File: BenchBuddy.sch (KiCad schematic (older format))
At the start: 0 parts

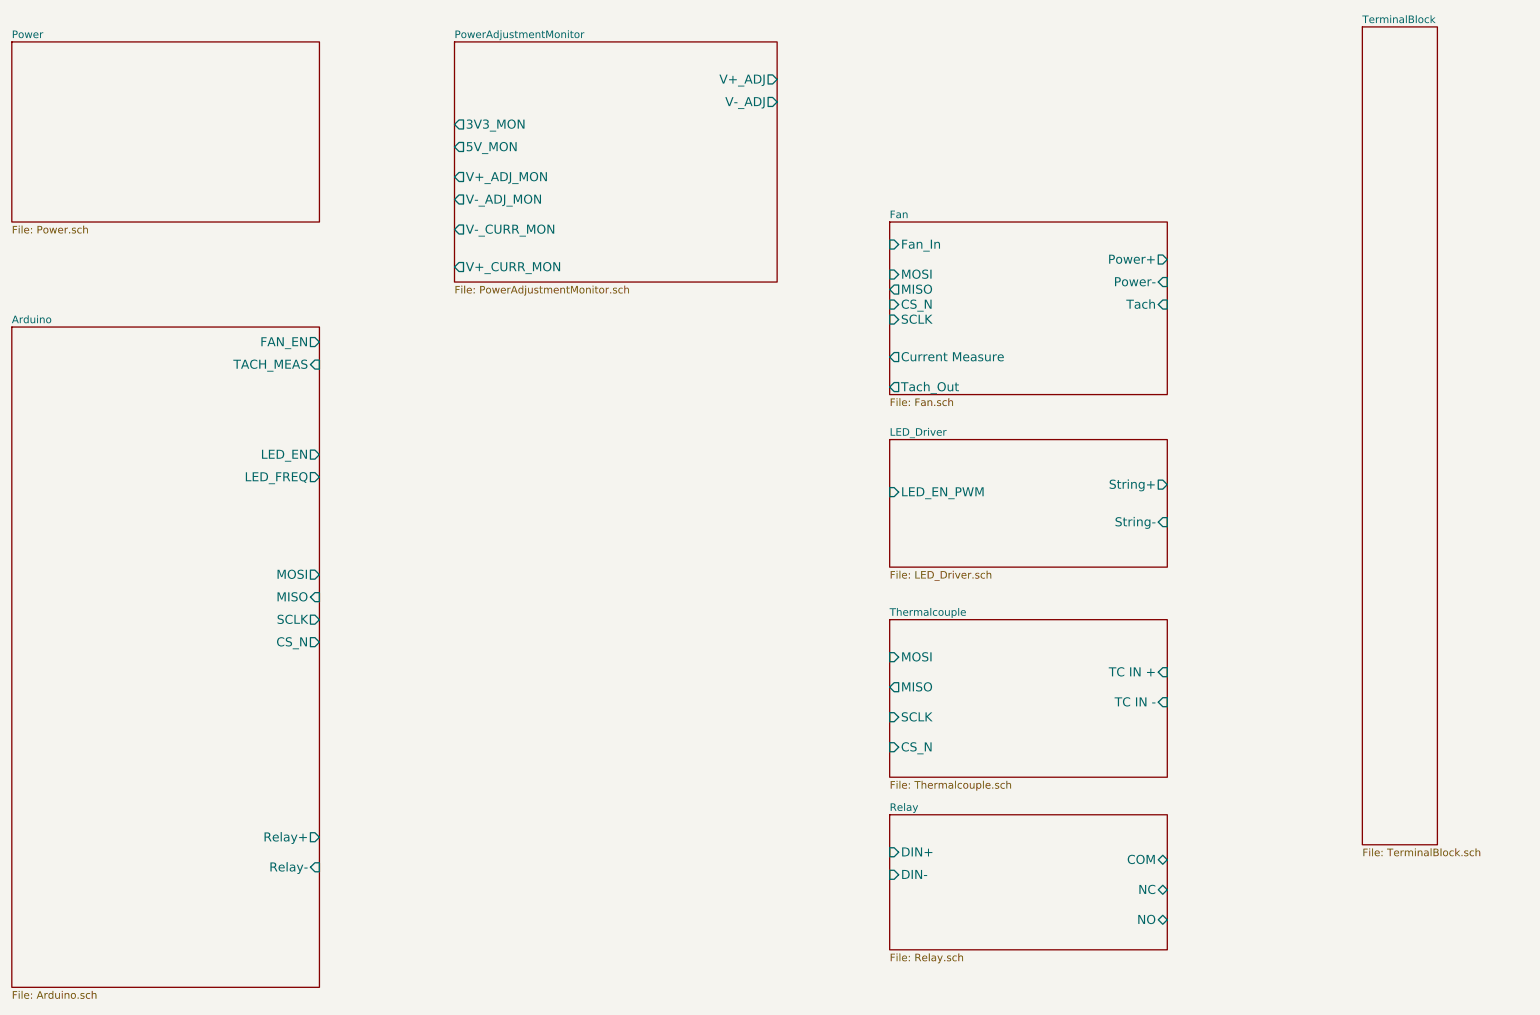
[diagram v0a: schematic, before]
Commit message: arduino module / hooking things up
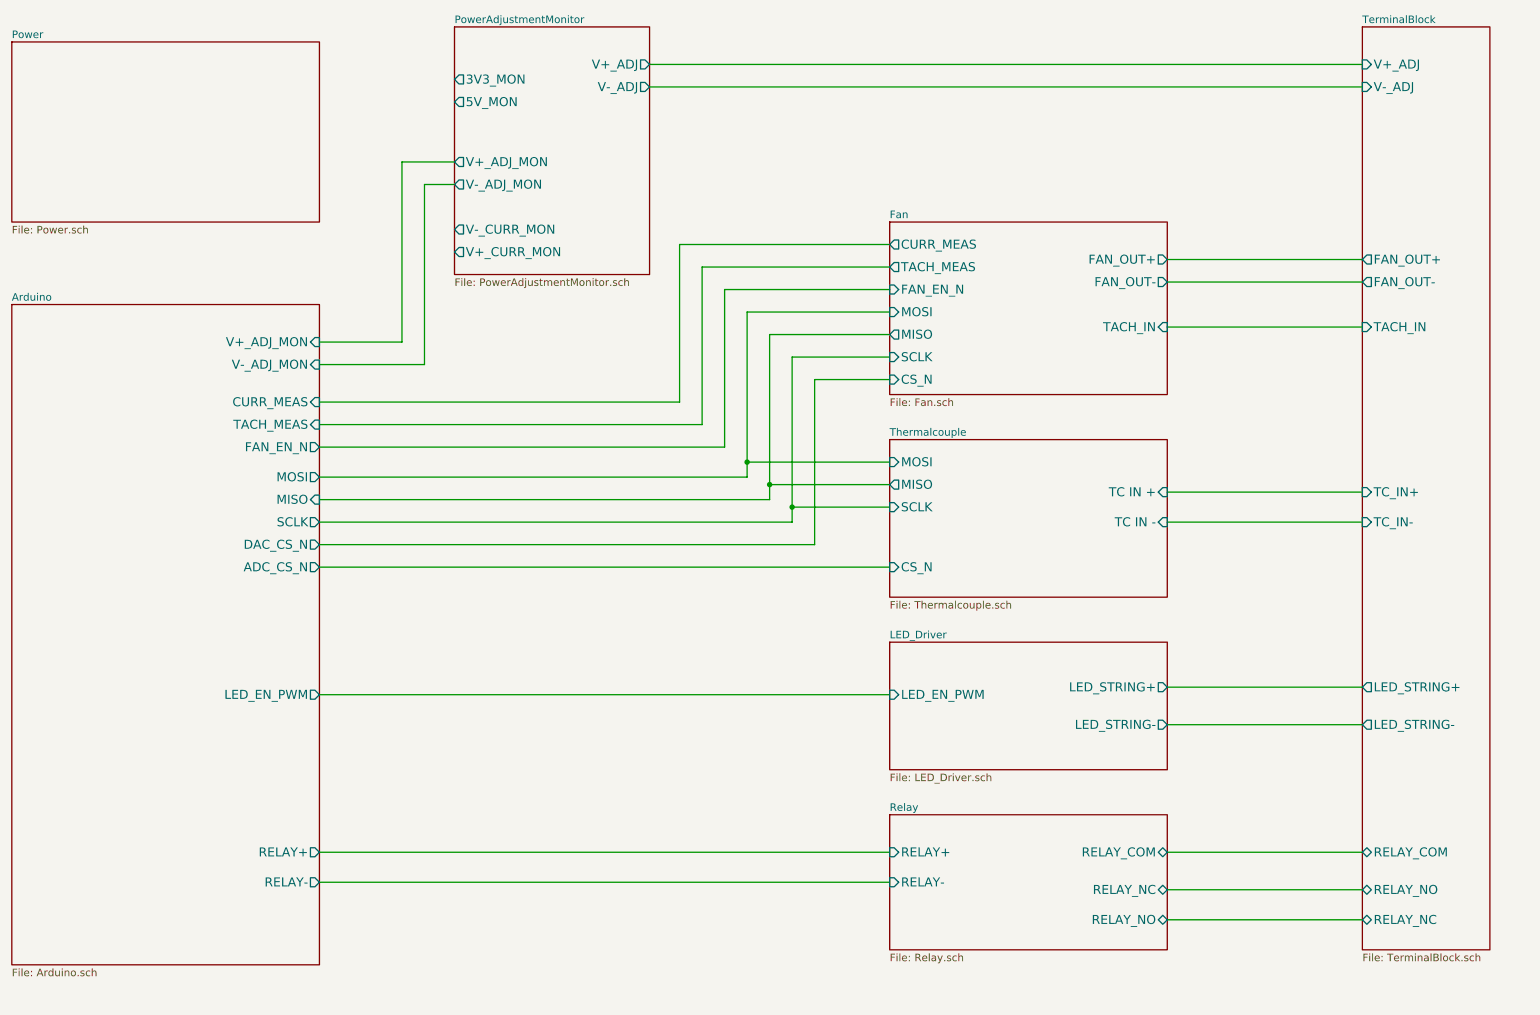
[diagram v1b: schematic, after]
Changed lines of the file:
@@
 $EndDescr
-$Sheet
-S 1250 2800 2050 4400
-U 52EEB005
-F0 "Arduino" 50
-F1 "Arduino.sch" 50
-F2 "Relay+" O R 3300 6200 60
-F3 "Relay-" I R 3300 6400 60
-F4 "MOSI" O R 3300 4450 60
-F5 "MISO" I R 3300 4600 60
-F6 "SCLK" O R 3300 4750 60
-F7 "CS_N" O R 3300 4900 60
-F8 "LED_EN" O R 3300 3650 60
-F9 "LED_FREQ" O R 3300 3800 60
-F10 "FAN_EN" O R 3300 2900 60
-F11 "TACH_MEAS" I R 3300 3050 60
-$EndSheet
 $Sheet
 S 7100 6050 1850 900
@@
 F0 "Relay" 50
 F1 "Relay.sch" 50
-F2 "DIN+" I L 7100 6300 60
-F3 "DIN-" I L 7100 6450 60
-F4 "NC" B R 8950 6550 60
-F5 "NO" B R 8950 6750 60
-F6 "COM" B R 8950 6350 60
+F2 "RELAY_NC" B R 8950 6550 60
+F3 "RELAY_NO" B R 8950 6750 60
+F4 "RELAY_COM" B R 8950 6300 60
+F5 "RELAY+" I L 7100 6300 60
+F6 "RELAY-" I L 7100 6500 60
 $EndSheet
 $Sheet
@@
 $EndSheet
 $Sheet
-S 7100 3550 1850 850
+S 7100 4900 1850 850
 U 52EEB0B1
 F0 "LED_Driver" 50
 F1 "LED_Driver.sch" 50
-F2 "String+" O R 8950 3850 60
-F3 "String-" I R 8950 4100 60
-F4 "LED_EN_PWM" I L 7100 3900 60
+F2 "LED_EN_PWM" I L 7100 5250 60
+F3 "LED_STRING+" O R 8950 5200 60
+F4 "LED_STRING-" O R 8950 5450 60
+$EndSheet
+$Sheet
+S 10250 800  850  6150
+U 52EEB0FB
+F0 "TerminalBlock" 50
+F1 "TerminalBlock.sch" 50
+F2 "V+_ADJ" I L 10250 1050 60
+F3 "V-_ADJ" I L 10250 1200 60
+F4 "FAN_OUT+" O L 10250 2350 60
+F5 "TACH_IN" I L 10250 2800 60
+F6 "FAN_OUT-" O L 10250 2500 60
+F7 "LED_STRING+" O L 10250 5200 60
+F8 "LED_STRING-" O L 10250 5450 60
+F9 "TC_IN+" I L 10250 3900 60
+F10 "TC_IN-" I L 10250 4100 60
+F11 "RELAY_COM" B L 10250 6300 60
+F12 "RELAY_NO" B L 10250 6550 60
+F13 "RELAY_NC" B L 10250 6750 60
+$EndSheet
+$Sheet
+S 7100 3550 1850 1050
+U 52EEB050
+F0 "Thermalcouple" 50
+F1 "Thermalcouple.sch" 50
+F2 "TC IN +" I R 8950 3900 60
+F3 "TC IN -" I R 8950 4100 60
+F4 "MOSI" I L 7100 3700 60
+F5 "MISO" O L 7100 3850 60
+F6 "SCLK" I L 7100 4000 60
+F7 "CS_N" I L 7100 4400 60
+$EndSheet
+$Sheet
+S 4200 800  1300 1650
+U 52F3A754
+F0 "PowerAdjustmentMonitor" 50
+F1 "PowerAdjustmentMonitor.sch" 50
+F2 "V+_ADJ" O R 5500 1050 60
+F3 "V-_ADJ" O R 5500 1200 60
+F4 "3V3_MON" O L 4200 1150 60
+F5 "5V_MON" O L 4200 1300 60
+F6 "V+_ADJ_MON" O L 4200 1700 60
+F7 "V-_ADJ_MON" O L 4200 1850 60
+F8 "V+_CURR_MON" O L 4200 2300 60
+F9 "V-_CURR_MON" O L 4200 2150 60
 $EndSheet
 $Sheet
@@
 F0 "Fan" 50
 F1 "Fan.sch" 50
-F2 "Power+" O R 8950 2350 60
-F3 "Power-" I R 8950 2500 60
-F4 "Tach" I R 8950 2650 60
-F5 "Tach_Out" O L 7100 3200 60
-F6 "Fan_In" I L 7100 2250 60
-F7 "Current Measure" O L 7100 3000 60
-F8 "MOSI" I L 7100 2450 60
-F9 "MISO" O L 7100 2550 60
-F10 "CS_N" I L 7100 2650 60
-F11 "SCLK" I L 7100 2750 60
-$EndSheet
-$Sheet
-S 10250 800  500  5450
-U 52EEB0FB
-F0 "TerminalBlock" 50
-F1 "TerminalBlock.sch" 50
-$EndSheet
-$Sheet
-S 7100 4750 1850 1050
-U 52EEB050
-F0 "Thermalcouple" 50
-F1 "Thermalcouple.sch" 50
-F2 "TC IN +" I R 8950 5100 60
-F3 "TC IN -" I R 8950 5300 60
-F4 "MOSI" I L 7100 5000 60
-F5 "MISO" O L 7100 5200 60
-F6 "SCLK" I L 7100 5400 60
-F7 "CS_N" I L 7100 5600 60
-$EndSheet
-$Sheet
-S 4200 900  2150 1600
-U 52F3A754
-F0 "PowerAdjustmentMonitor" 50
-F1 "PowerAdjustmentMonitor.sch" 50
-F2 "V+_ADJ" O R 6350 1150 60
-F3 "V-_ADJ" O R 6350 1300 60
-F4 "3V3_MON" O L 4200 1450 60
-F5 "5V_MON" O L 4200 1600 60
-F6 "V+_ADJ_MON" O L 4200 1800 60
-F7 "V-_ADJ_MON" O L 4200 1950 60
-F8 "V+_CURR_MON" O L 4200 2400 60
-F9 "V-_CURR_MON" O L 4200 2150 60
-$EndSheet
+F2 "MOSI" I L 7100 2700 60
+F3 "MISO" O L 7100 2850 60
+F4 "CS_N" I L 7100 3150 60
+F5 "SCLK" I L 7100 3000 60
+F6 "FAN_OUT+" O R 8950 2350 60
+F7 "TACH_MEAS" O L 7100 2400 60
+F8 "FAN_EN_N" I L 7100 2550 60
+F9 "CURR_MEAS" O L 7100 2250 60
+F10 "TACH_IN" I R 8950 2800 60
+F11 "FAN_OUT-" O R 8950 2500 60
+$EndSheet
+$Sheet
+S 1250 2650 2050 4400
+U 52EEB005
+F0 "Arduino" 50
+F1 "Arduino.sch" 50
+F2 "MOSI" O R 3300 3800 60
+F3 "MISO" I R 3300 3950 60
+F4 "SCLK" O R 3300 4100 60
+F6 "TACH_MEAS" I R 3300 3450 60
+F7 "RELAY-" O R 3300 6500 60
+F8 "RELAY+" O R 3300 6300 60
+F9 "FAN_EN_N" O R 3300 3600 60
+F10 "CURR_MEAS" I R 3300 3300 60
+F11 "V+_ADJ_MON" I R 3300 2900 60
+F12 "V-_ADJ_MON" I R 3300 3050 60
+F13 "LED_EN_PWM" O R 3300 5250 60
+F14 "DAC_CS_N" O R 3300 4250 60
+F15 "ADC_CS_N" O R 3300 4400 60
+$EndSheet
+Wire Wire Line
+	5500 1050 10250 1050
+Wire Wire Line
+	5500 1200 10250 1200
+Wire Wire Line
+	8950 2350 10250 2350
+Wire Wire Line
+	10250 2500 8950 2500
+Wire Wire Line
+	8950 2800 10250 2800
+Wire Wire Line
+	8950 6300 10250 6300
+Wire Wire Line
+	10250 6550 8950 6550
+Wire Wire Line
+	8950 6750 10250 6750
+Wire Wire Line
+	3300 2900 3850 2900
+Wire Wire Line
+	3850 2900 3850 1700
+Wire Wire Line
+	3850 1700 4200 1700
+Wire Wire Line
+	3300 3050 4000 3050
+Wire Wire Line
+	4000 3050 4000 1850
+Wire Wire Line
+	4000 1850 4200 1850
+Wire Wire Line
+	3300 3300 5700 3300
+Wire Wire Line
+	5700 3300 5700 2250
+Wire Wire Line
+	5700 2250 7100 2250
+Wire Wire Line
+	3300 3450 5850 3450
+Wire Wire Line
+	5850 3450 5850 2400
+Wire Wire Line
+	5850 2400 7100 2400
+Wire Wire Line
+	7100 2550 6000 2550
+Wire Wire Line
+	6000 2550 6000 3600
+Wire Wire Line
+	6000 3600 3300 3600
+Wire Wire Line
+	3300 3800 6150 3800
+Wire Wire Line
+	6150 3800 6150 2700
+Wire Wire Line
+	6150 2700 7100 2700
+Wire Wire Line
+	6300 2850 7100 2850
+Wire Wire Line
+	6300 2850 6300 3950
+Wire Wire Line
+	6300 3950 3300 3950
+Wire Wire Line
+	3300 4100 6450 4100
+Wire Wire Line
+	6450 4100 6450 3000
+Wire Wire Line
+	6450 3000 7100 3000
+Wire Wire Line
+	7100 3150 6600 3150
+Wire Wire Line
+	6600 3150 6600 4250
+Wire Wire Line
+	6600 4250 3300 4250
+Wire Wire Line
+	3300 4400 7100 4400
+Wire Wire Line
+	7100 3700 6150 3700
+Connection ~ 6150 3700
+Wire Wire Line
+	7100 3850 6300 3850
+Connection ~ 6300 3850
+Wire Wire Line
+	7100 4000 6450 4000
+Connection ~ 6450 4000
+Wire Wire Line
+	3300 5250 7100 5250
+Wire Wire Line
+	7100 6300 3300 6300
+Wire Wire Line
+	3300 6500 7100 6500
+Wire Wire Line
+	8950 5450 10250 5450
+Wire Wire Line
+	10250 5200 8950 5200
+Wire Wire Line
+	8950 4100 10250 4100
+Wire Wire Line
+	10250 3900 8950 3900
 $EndSCHEMATC
